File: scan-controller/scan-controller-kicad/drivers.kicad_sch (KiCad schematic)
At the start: 54 parts, among them CN2 Motor, CN3 Fan, CN4 Lamp, Q1 CS12N06AE-G, U10 LGS5145, U11 MCP1416, U3 78L05, U4 DRV8871DDA, U6 TL431, U7 XL4015, U8 LM358

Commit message: reassigned customfootprints to now gobal library
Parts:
- TP14, TP15, TP16, TP17, TP18, TP9: footprint Peacemans_Footprints:TestPoint_THTPad_1.5x1.5mm_Drill0.7mm_named -> Peacemans_Teile:TestPoint_THTPad_1.5x1.5mm_Drill0.7mm_named
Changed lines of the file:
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@@
 			)
 		)
-		(property "Footprint" "Peacemans_Footprints:TestPoint_THTPad_1.5x1.5mm_Drill0.7mm_named"
+		(property "Footprint" "Peacemans_Teile:TestPoint_THTPad_1.5x1.5mm_Drill0.7mm_named"
 			(at 227.965 134.62 0)
 			(effects
@@
 			)
 		)
-		(property "Footprint" "Peacemans_Footprints:TestPoint_THTPad_1.5x1.5mm_Drill0.7mm_named"
+		(property "Footprint" "Peacemans_Teile:TestPoint_THTPad_1.5x1.5mm_Drill0.7mm_named"
 			(at 258.445 34.925 0)
 			(effects
@@
 			)
 		)
-		(property "Footprint" "Peacemans_Footprints:TestPoint_THTPad_1.5x1.5mm_Drill0.7mm_named"
+		(property "Footprint" "Peacemans_Teile:TestPoint_THTPad_1.5x1.5mm_Drill0.7mm_named"
 			(at 197.485 83.82 0)
 			(effects
@@
 			)
 		)
-		(property "Footprint" "Peacemans_Footprints:TestPoint_THTPad_1.5x1.5mm_Drill0.7mm_named"
+		(property "Footprint" "Peacemans_Teile:TestPoint_THTPad_1.5x1.5mm_Drill0.7mm_named"
 			(at 266.065 53.34 0)
 			(effects
@@
 			)
 		)
-		(property "Footprint" "Peacemans_Footprints:TestPoint_THTPad_1.5x1.5mm_Drill0.7mm_named"
+		(property "Footprint" "Peacemans_Teile:TestPoint_THTPad_1.5x1.5mm_Drill0.7mm_named"
 			(at 267.335 34.925 0)
 			(effects
@@
 			)
 		)
-		(property "Footprint" "Peacemans_Footprints:TestPoint_THTPad_1.5x1.5mm_Drill0.7mm_named"
+		(property "Footprint" "Peacemans_Teile:TestPoint_THTPad_1.5x1.5mm_Drill0.7mm_named"
 			(at 228.6 116.205 0)
 			(effects

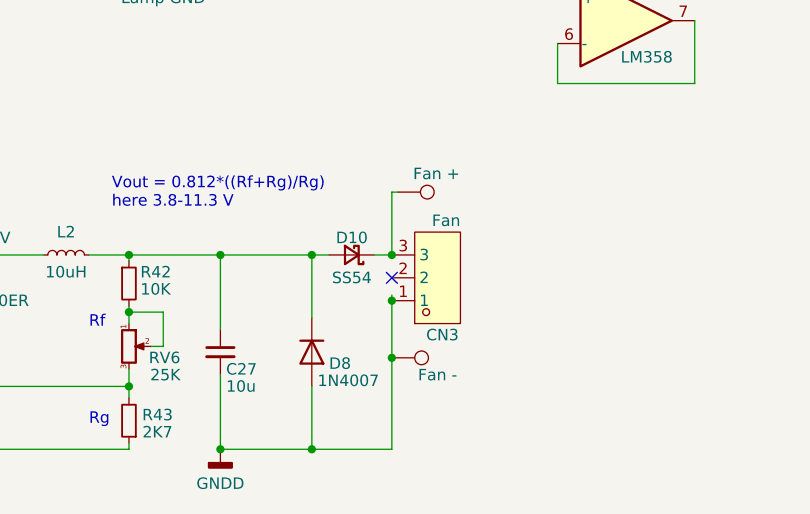
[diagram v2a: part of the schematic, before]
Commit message: Massive rearrangement :)
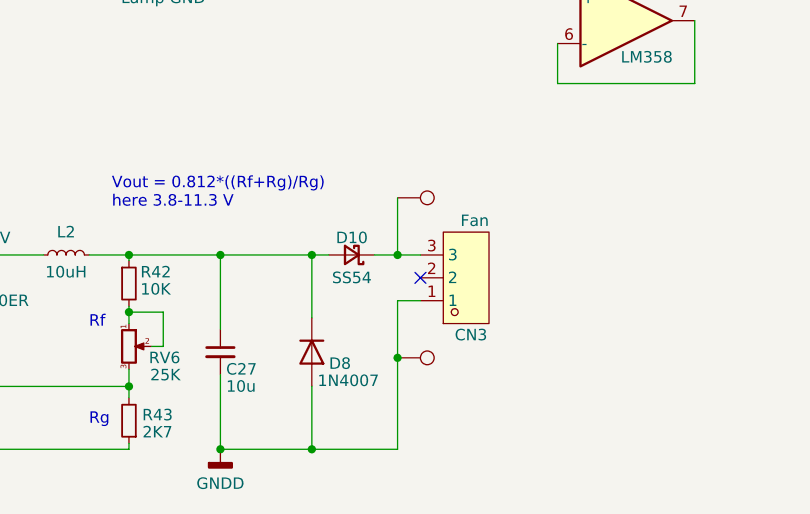
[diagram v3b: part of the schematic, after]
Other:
- moved on the sheet: CN3
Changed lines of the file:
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@@
 	)
 	(junction
-		(at 227.965 123.19)
+		(at 237.49 46.355)
 		(diameter 0)
 		(color 0 0 0 0)
 	)
 	(junction
-		(at 237.49 46.355)
+		(at 182.245 83.82)
 		(diameter 0)
 		(color 0 0 0 0)
 	)
 	(junction
-		(at 182.245 83.82)
+		(at 193.675 83.82)
 		(diameter 0)
 		(color 0 0 0 0)
 	)
 	(junction
-		(at 193.675 83.82)
+		(at 228.6 129.54)
 		(diameter 0)
 		(color 0 0 0 0)
@@
 	)
 	(junction
-		(at 227.965 129.54)
-		(diameter 0)
-		(color 0 0 0 0)
-	)
-	(junction
 		(at 208.915 118.11)
 		(diameter 0)
@@
 	)
 	(junction
-		(at 227.965 118.11)
+		(at 219.075 139.7)
 		(diameter 0)
 		(color 0 0 0 0)
 	)
 	(junction
-		(at 219.075 139.7)
+		(at 170.18 76.2)
 		(diameter 0)
 		(color 0 0 0 0)
 	)
 	(junction
-		(at 170.18 76.2)
+		(at 228.6 118.11)
 		(diameter 0)
 		(color 0 0 0 0)
 	)
 	(no_connect
-		(at 227.965 120.65)
+		(at 231.14 120.65)
 	)
 	(wire
@@
 	(wire
 		(pts
+			(xy 231.14 118.11) (xy 228.6 118.11)
+		)
+		(stroke
+			(width 0)
+			(type default)
+		)
+	)
+	(wire
+		(pts
 			(xy 166.37 60.325) (xy 165.735 60.325)
 		)
@@
 	(wire
 		(pts
-			(xy 227.965 111.125) (xy 227.965 118.11)
+			(xy 228.6 111.76) (xy 228.6 118.11)
 		)
 		(stroke
@@
 	(wire
 		(pts
-			(xy 226.06 118.11) (xy 227.965 118.11)
+			(xy 226.06 118.11) (xy 228.6 118.11)
 		)
 		(stroke
@@
 	(wire
 		(pts
-			(xy 227.965 123.19) (xy 227.965 129.54)
-		)
-		(stroke
-			(width 0)
-			(type default)
-		)
-	)
-	(wire
-		(pts
 			(xy 147.955 40.64) (xy 147.955 39.37)
 		)
@@
 	(wire
 		(pts
-			(xy 227.965 122.555) (xy 227.965 123.19)
+			(xy 228.6 123.19) (xy 228.6 129.54)
 		)
 		(stroke
@@
 	(wire
 		(pts
-			(xy 227.965 129.54) (xy 227.965 139.7)
+			(xy 228.6 129.54) (xy 228.6 139.7)
 		)
 		(stroke
@@
 	(wire
 		(pts
-			(xy 228.6 111.125) (xy 227.965 111.125)
-		)
-		(stroke
-			(width 0)
-			(type default)
-		)
-	)
-	(wire
-		(pts
 			(xy 177.8 83.82) (xy 182.245 83.82)
 		)
@@
 	(wire
 		(pts
-			(xy 227.965 139.7) (xy 219.075 139.7)
+			(xy 228.6 139.7) (xy 219.075 139.7)
 		)
 		(stroke
@@
 	(wire
 		(pts
+			(xy 228.6 123.19) (xy 231.14 123.19)
+		)
+		(stroke
+			(width 0)
+			(type default)
+		)
+	)
+	(wire
+		(pts
 			(xy 250.825 43.815) (xy 250.825 48.26)
 		)
@@
 	(symbol
 		(lib_id "easyeda2kicad:KF141R-2.54-3P")
-		(at 233.045 120.65 0)
+		(at 236.22 120.65 0)
 		(mirror x)
 		(unit 1)
@@
 		(dnp no)
 		(property "Reference" "CN3"
-			(at 231.775 127 0)
+			(at 234.95 127 0)
 			(effects
 				(font
@@
 		)
 		(property "Value" "Fan"
-			(at 232.41 114.3 0)
+			(at 235.585 114.3 0)
 			(effects
 				(font
@@
 		)
 		(property "Footprint" "easyeda2kicad:CONN-TH_3P-P2.54_DIBO_DB141R-2.54-3P"
-			(at 233.045 110.49 0)
+			(at 236.22 110.49 0)
 			(effects
 				(font
@@
 		)
 		(property "Datasheet" "https://lcsc.com/product-detail/New-Quadratic-Unclassified-Data_Cixi-Kefa-Elec-KF141R-2-54-3P_C475125.html"
-			(at 233.045 107.95 0)
+			(at 236.22 107.95 0)
 			(effects
 				(font
@@
 		)
 		(property "Description" ""
-			(at 233.045 120.65 0)
+			(at 236.22 120.65 0)
 			(effects
 				(font
@@
 		)
 		(property "LCSC Part" ""
-			(at 233.045 105.41 0)
+			(at 236.22 105.41 0)
 			(effects
 				(font
@@
 		)
 		(property "LCSC" "C2898755"
-			(at 233.045 120.65 0)
+			(at 236.22 120.65 0)
 			(effects
 				(font
@@
 		)
 		(property "Inventory" ""
-			(at 233.045 120.65 0)
+			(at 236.22 120.65 0)
 			(effects
 				(font
@@
 		)
 		(property "Sim.Device" "C475125"
-			(at 233.045 120.65 0)
+			(at 236.22 120.65 0)
 			(effects
 				(font
@@
 	(symbol
 		(lib_id "Peacemans_Teile:TestPoint_named")
-		(at 227.965 129.54 270)
+		(at 228.6 129.54 270)
 		(unit 1)
 		(exclude_from_sim no)
@@
 		(dnp no)
 		(property "Reference" "TP17"
-			(at 234.823 129.54 0)
+			(at 235.458 129.54 0)
 			(effects
 				(font
@@
 		)
 		(property "Value" "TestPoint"
-			(at 233.045 129.54 0)
+			(at 233.68 129.54 0)
 			(effects
 				(font
@@
 		)
 		(property "Footprint" "Peacemans_Teile:TestPoint_THTPad_1.5x1.5mm_Drill0.7mm_named"
-			(at 227.965 134.62 0)
+			(at 228.6 134.62 0)
 			(effects
 				(font
@@
 		)
 		(property "Datasheet" "~"
-			(at 227.965 134.62 0)
+			(at 228.6 134.62 0)
 			(effects
 				(font
@@
 		)
 		(property "Description" ""
-			(at 227.965 129.54 0)
+			(at 228.6 129.54 0)
 			(effects
 				(font
@@
 		)
 		(property "TP_Label" "Fan -"
-			(at 233.045 131.445 90)
+			(at 233.68 131.445 90)
 			(effects
 				(font
 					(size 1.27 1.27)
 				)
+				(hide yes)
 			)
 		)
@@
 	(symbol
 		(lib_id "Peacemans_Teile:TestPoint_named")
-		(at 228.6 111.125 270)
+		(at 228.6 111.76 270)
 		(unit 1)
 		(exclude_from_sim no)
@@
 		(dnp no)
 		(property "Reference" "TP18"
-			(at 235.458 111.125 0)
+			(at 235.458 111.76 0)
 			(effects
 				(font
@@
 		)
 		(property "Value" "TestPoint"
-			(at 233.68 111.125 0)
+			(at 233.68 111.76 0)
 			(effects
 				(font
@@
 		)
 		(property "Footprint" "Peacemans_Teile:TestPoint_THTPad_1.5x1.5mm_Drill0.7mm_named"
-			(at 228.6 116.205 0)
+			(at 228.6 116.84 0)
 			(effects
 				(font
@@
 		)
 		(property "Datasheet" "~"
-			(at 228.6 116.205 0)
+			(at 228.6 116.84 0)
 			(effects
 				(font
@@
 		)
 		(property "Description" ""
-			(at 228.6 111.125 0)
+			(at 228.6 111.76 0)
 			(effects
 				(font
@@
 		)
 		(property "TP_Label" "Fan +"
-			(at 232.918 109.093 90)
+			(at 232.918 109.728 90)
 			(effects
 				(font
 					(size 1.27 1.27)
 				)
+				(hide yes)
 			)
 		)
